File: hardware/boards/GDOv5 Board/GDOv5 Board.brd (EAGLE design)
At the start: 100 x 80 mm, 27 parts, among them IC1 DS1820, IC2 REG1117, J1 DCJ0202

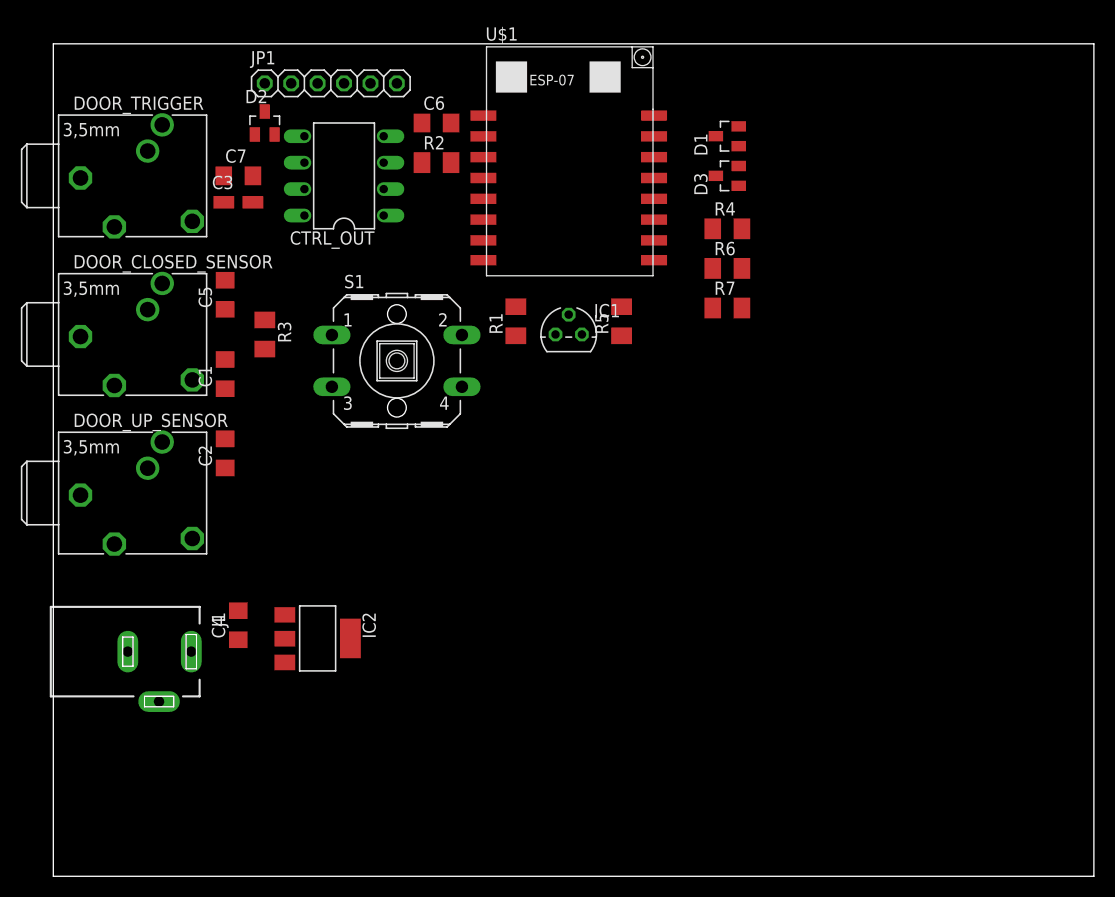
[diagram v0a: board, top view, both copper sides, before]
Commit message: Updating routing and layout
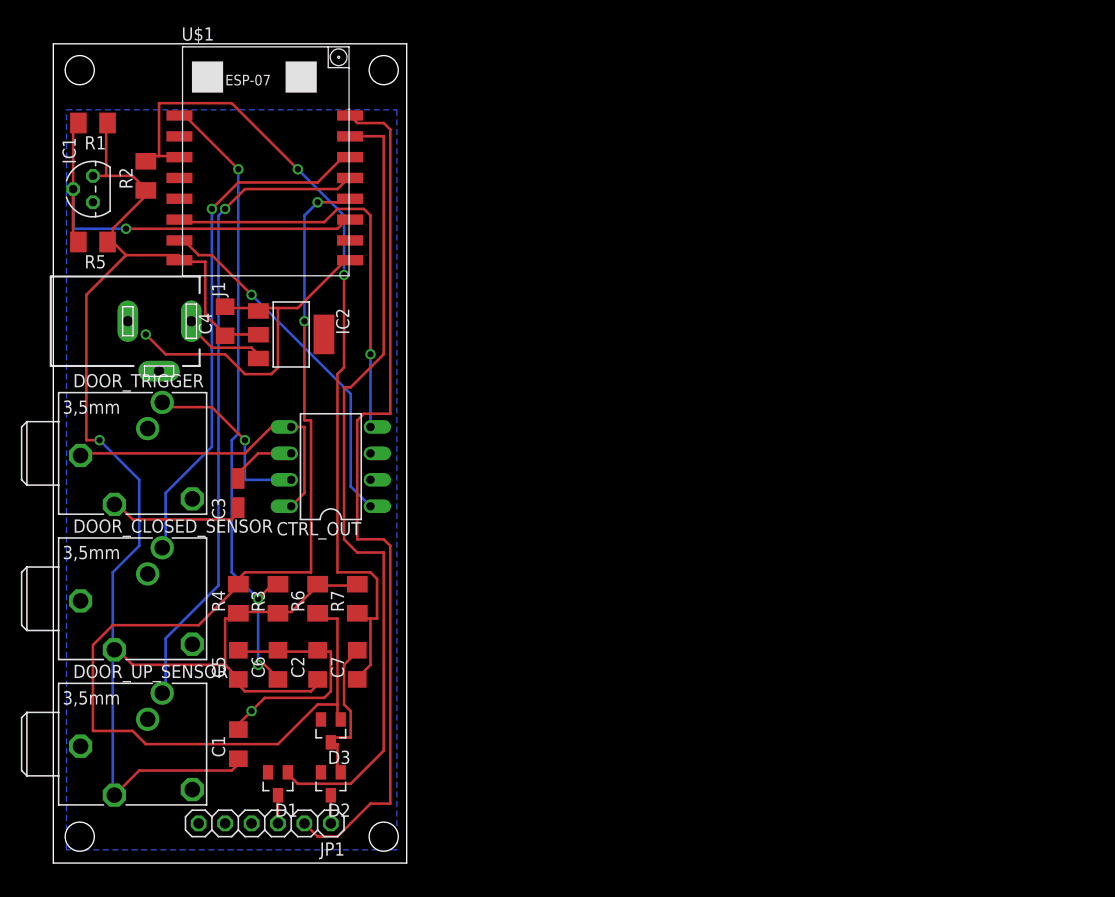
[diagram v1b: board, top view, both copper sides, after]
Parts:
- removed S1: (no value), adafruit:B3F-40XX
- moved D1 75.7 mm to (21.6, 8.89), turned to 180 degrees
- moved JP1 71.4 mm to (20.3, 5.08), turned to 180 degrees
- moved D3 65.5 mm to (26.7, 14.0), turned to 180 degrees
- moved D2 63.8 mm to (26.7, 8.89), turned to 180 degrees
- moved R4 58.9 mm to (17.8, 26.7), turned to 90 degrees
- moved C6 54.3 mm to (21.6, 20.3), turned to 90 degrees
- moved R5 51.4 mm to (3.81, 61.0), turned to 180 degrees
- moved R6 50.6 mm to (25.4, 26.7), turned to 90 degrees
- moved C7 48.4 mm to (29.2, 20.3), turned to 90 degrees
- moved IC1 47.8 mm to (3.81, 66.0), turned to 90 degrees
- moved R7 45.2 mm to (29.2, 26.7), turned to 90 degrees
- moved R1 44.9 mm to (3.81, 72.4), turned to 180 degrees
- moved C1 35.6 mm to (17.8, 12.7)
- moved C5 35.6 mm to (17.8, 20.3)
- moved J1 31.8 mm to (10.2, 53.3)
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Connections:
- net GND: no longer S1.3, S1.4
- net RESET: no longer S1.1, S1.2
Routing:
- net +3.3V: track 0.00 -> 151.3 mm, vias 0 -> 1
- net ARD0_FLASH: track 0.00 -> 110.3 mm, vias 0 -> 2
- net TXD: track 0.00 -> 84.9 mm
- net ENABLE: track 0.00 -> 82.3 mm, vias 0 -> 2
- net RXD: track 0.00 -> 78.3 mm
- net ARD05: track 0.00 -> 62.3 mm, vias 0 -> 1
- net RESET: track 0.00 -> 61.8 mm, vias 0 -> 3
- net GND: track 0.00 -> 58.4 mm, vias 0 -> 2
- net ARD04: track 0.00 -> 50.0 mm, vias 0 -> 1
- net ARD02: track 0.00 -> 43.2 mm, vias 0 -> 1
- net ARD12: track 0.00 -> 39.5 mm, vias 0 -> 1
- net ARD13: track 0.00 -> 34.1 mm, vias 0 -> 1
- net CTRL-: track 0.00 -> 30.7 mm
- net DOOR+: track 0.00 -> 17.8 mm, vias 0 -> 1
- net N$1: track 0.00 -> 15.2 mm
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- added copper zone on layer 16, net GND
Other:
- board size 100 x 80 mm -> 34 x 78.7 mm
